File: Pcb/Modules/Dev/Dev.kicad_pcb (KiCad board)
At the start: 2 copper layers, 50.8 x 50.8 mm, 10 parts, among them J1 JACK_STEREO, J2 JACK_RJ45, P1 CONN_02X04, P2 CONN_02X04, Q1 Q_NMOS_GSD

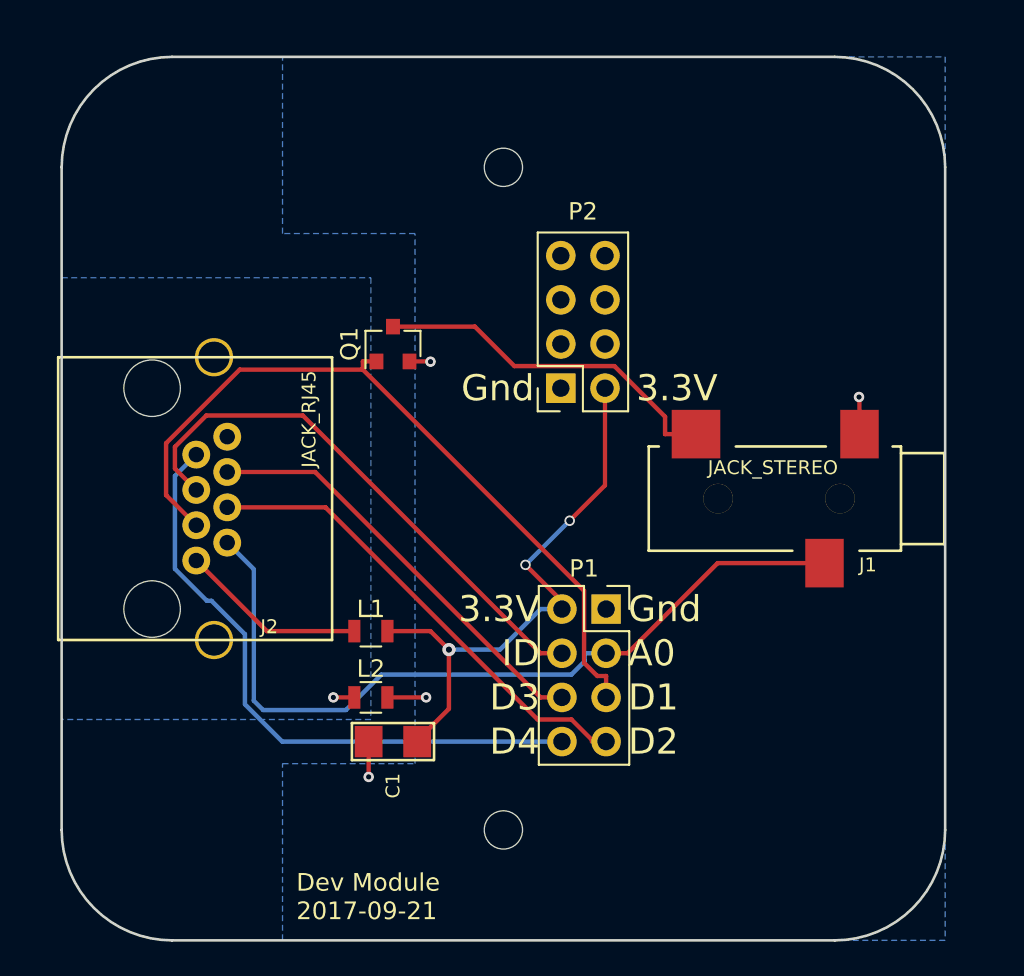
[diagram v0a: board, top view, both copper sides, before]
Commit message: Update dev module pcb
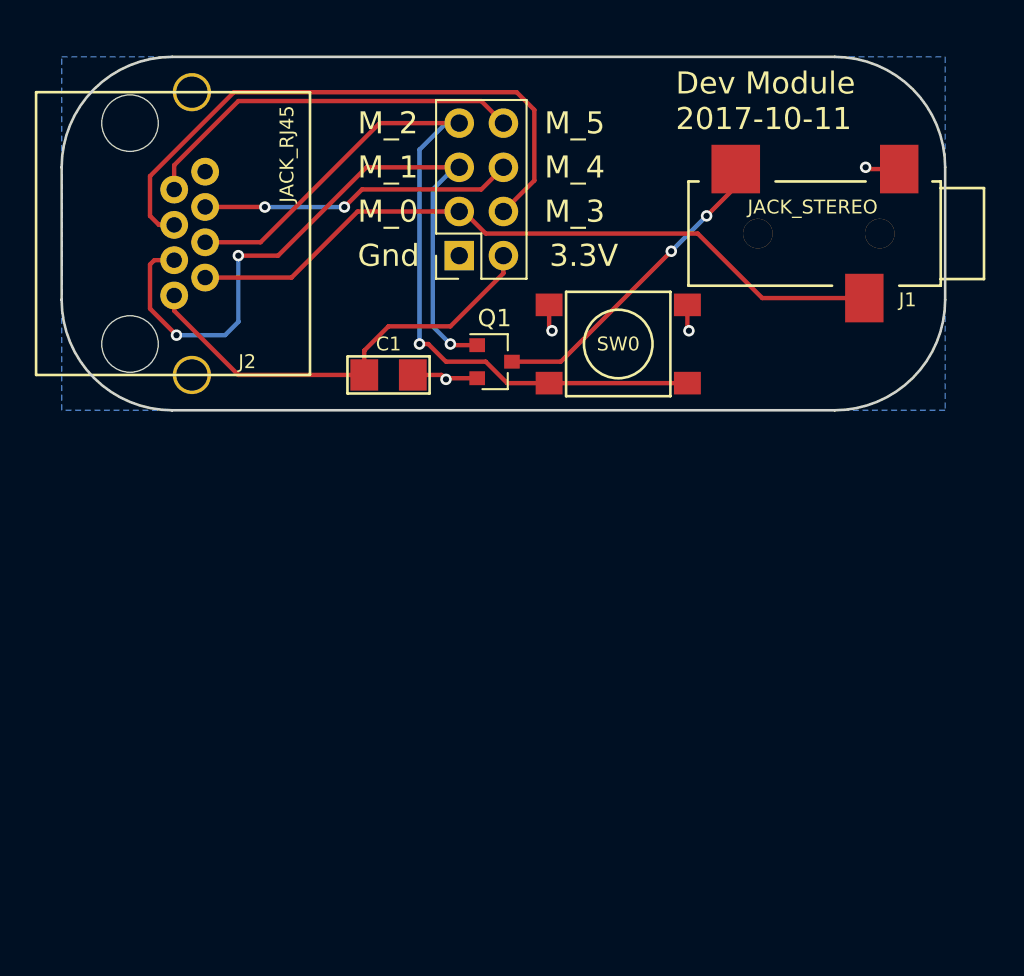
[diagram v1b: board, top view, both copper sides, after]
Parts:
- removed L1, L2: Ferrite_Bead, Resistors_SMD:R_0805
- removed P2: CONN_02X04, Socket_Strips:Socket_Strip_Straight_2x04_Pitch2.54mm
- removed REF**, REF**1: MountingHole_2.2mm_M2, Mounting_Holes:MountingHole_2.2mm_M2
- added SW0: SW_TACTILE, CA6:PTS645, F.Cu at (57.4, 41.9)
- moved P1 22.0 mm to (48.3, 36.8), turned to 180 degrees
- moved C1 21.1 mm to (44.2, 43.7), turned to 180 degrees
- moved J1 15.4 mm to (75.9, 35.6)
- moved J2 15.3 mm to (31.8, 35.6)
- moved Q1 5.93 mm to (50.3, 42.9), turned to 0 degrees
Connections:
- net /A0 renamed /M_0
- net /D1 renamed /M_1
- net /D2 renamed /M_2
- net /D3 renamed /M_4
- net /D4 renamed /M_5
- net /ID renamed /M_3
- J2 pad 1: Net-(J2-Pad1) -> 3V3
- J2 pad 8: Net-(J2-Pad8) -> GND
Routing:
- net /M_2: track 27.5 -> 47.9 mm, vias 0 -> 1
- net /M_5: track 35.8 -> 22.4 mm
- net Net-(J2-Pad1): track 10.8 -> 0.00 mm
- net 3V3: track 33.0 -> 25.6 mm, vias 3 -> 0
- net /M_4: track 24.6 -> 18.1 mm, vias 0 -> 2
- net /M_0: track 46.5 -> 41.5 mm
- net /M_3: track 31.6 -> 35.0 mm
- net /M_1: track 44.7 -> 41.6 mm, vias 0 -> 3
- net Net-(J1-Pad2): track 20.6 -> 18.1 mm, vias 0 -> 2
- net GND: track 7.62 -> 8.89 mm
- net Net-(J2-Pad8): track 1.21 -> 0.00 mm, vias 1 -> 0
- removed copper zone on B.Cu, net Net-(J2-Pad8)
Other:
- board size 50.8 x 50.8 mm -> 50.8 x 20.3 mm
- net class Default: clearance 0.2 -> 0.2032; trace_width 0.25 -> 0.254; via_dia 0.6 -> 0.6604; via_drill 0.4 -> 0.3556
- rule trace_clearance: 0.2 -> 0.2032
- board text added: "Dev Module 2017-10-11"
- board text added: "M_0"
- board text added: "M_1"
- board text added: "M_2"
- board text added: "M_3"
- board text added: "M_4"
- board text added: "M_5"
- board text removed: "A0"
- board text removed: "D1"
- board text removed: "D2"
- board text removed: "D3"
- board text removed: "D4"
- board text removed: "Dev Module 2017-09-21"
- board text removed: "ID"

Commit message: Update dev pcb layout
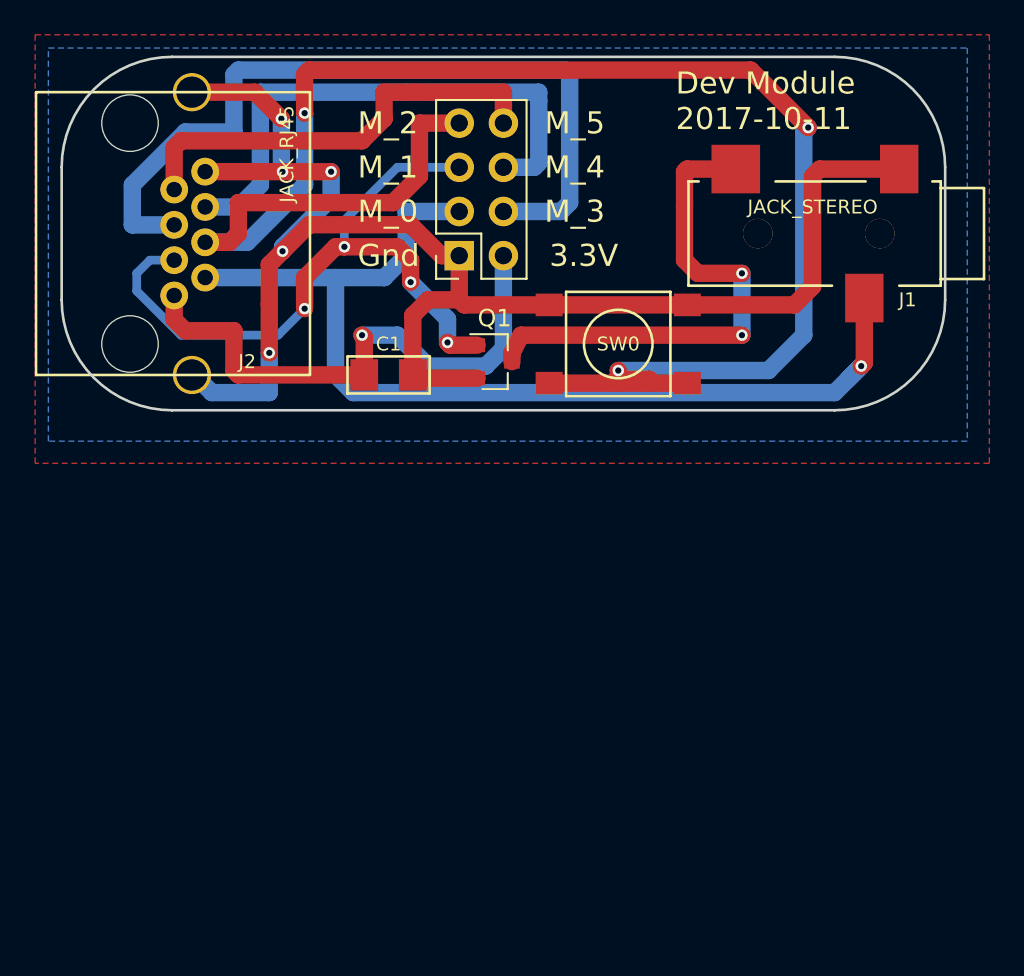
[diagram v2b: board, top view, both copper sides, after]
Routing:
- net GND: track 8.89 -> 91.8 mm, vias 4 -> 5
- net /M_2: track 47.9 -> 98.5 mm, vias 1 -> 3
- net /M_0: track 41.5 -> 59.6 mm, vias 0 -> 1
- net /M_4: track 18.1 -> 31.2 mm, vias 2 -> 0
- net Net-(J1-Pad2): track 18.1 -> 29.6 mm
- net /M_3: track 35.0 -> 46.0 mm
- net 3V3: track 25.6 -> 31.9 mm, vias 0 -> 1
- net /M_5: track 22.4 -> 25.3 mm
- net /M_1: track 41.6 -> 40.5 mm, vias 3 -> 4
- added copper zone on F.Cu, net GND
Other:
- net class Default: trace_width 0.254 -> 1
